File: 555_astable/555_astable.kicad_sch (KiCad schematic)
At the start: 10 parts, among them J1 Conn_01x02, J2 Conn_01x03, J3 Conn_01x02, SW1 SW_SPST, U1 NE555P

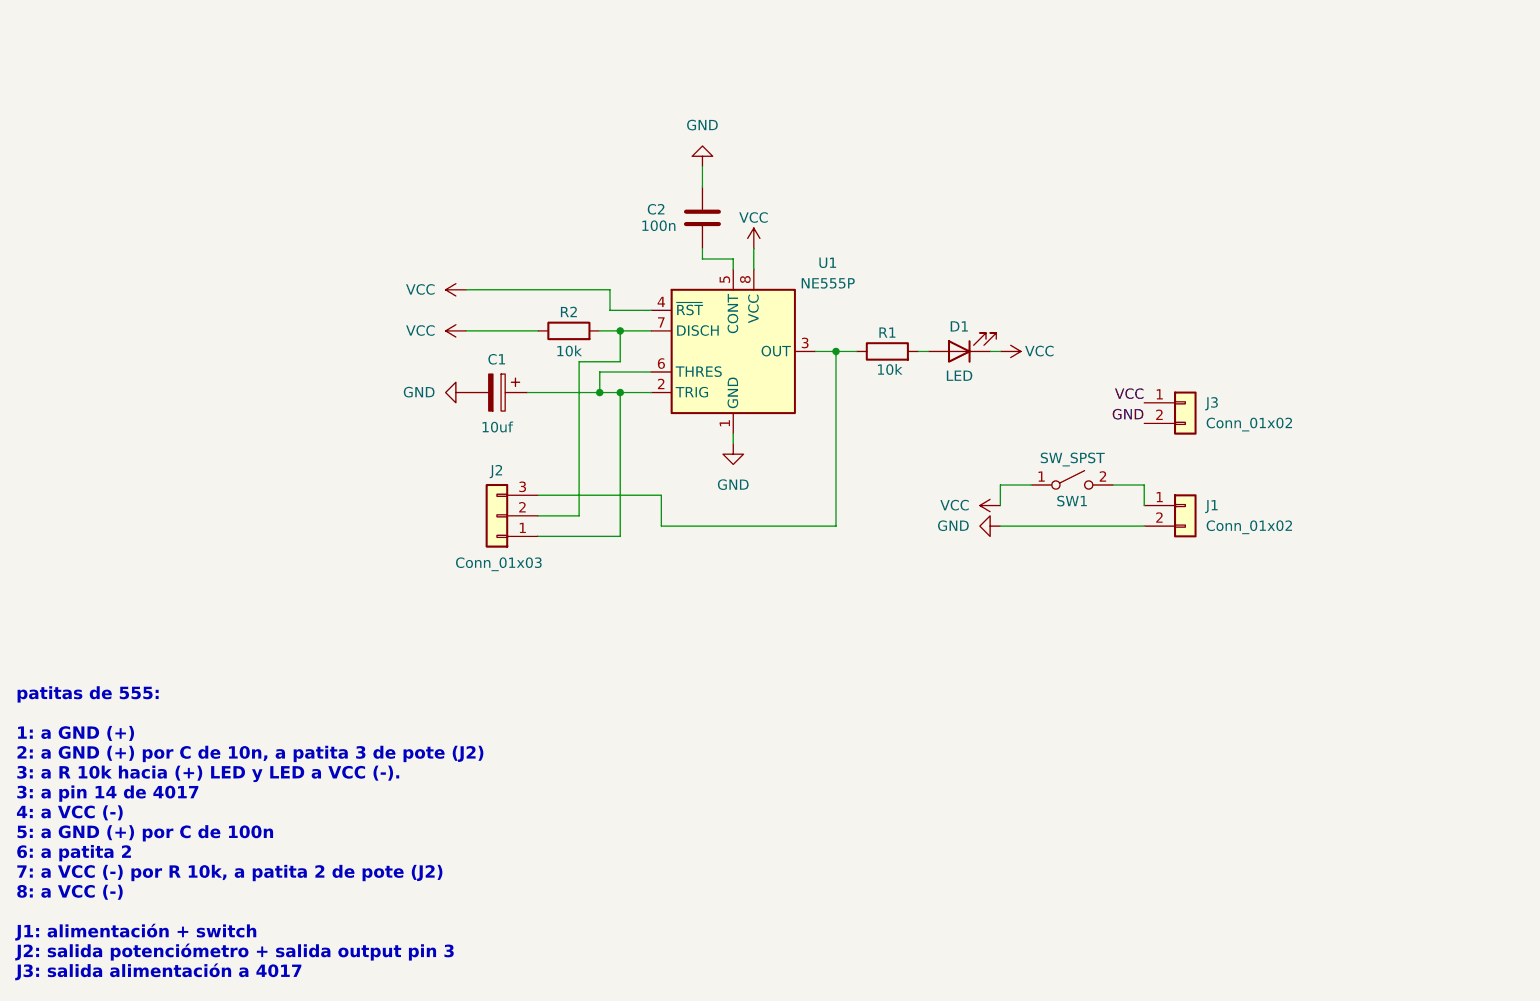
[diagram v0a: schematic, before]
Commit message: nueva version corregida de sch
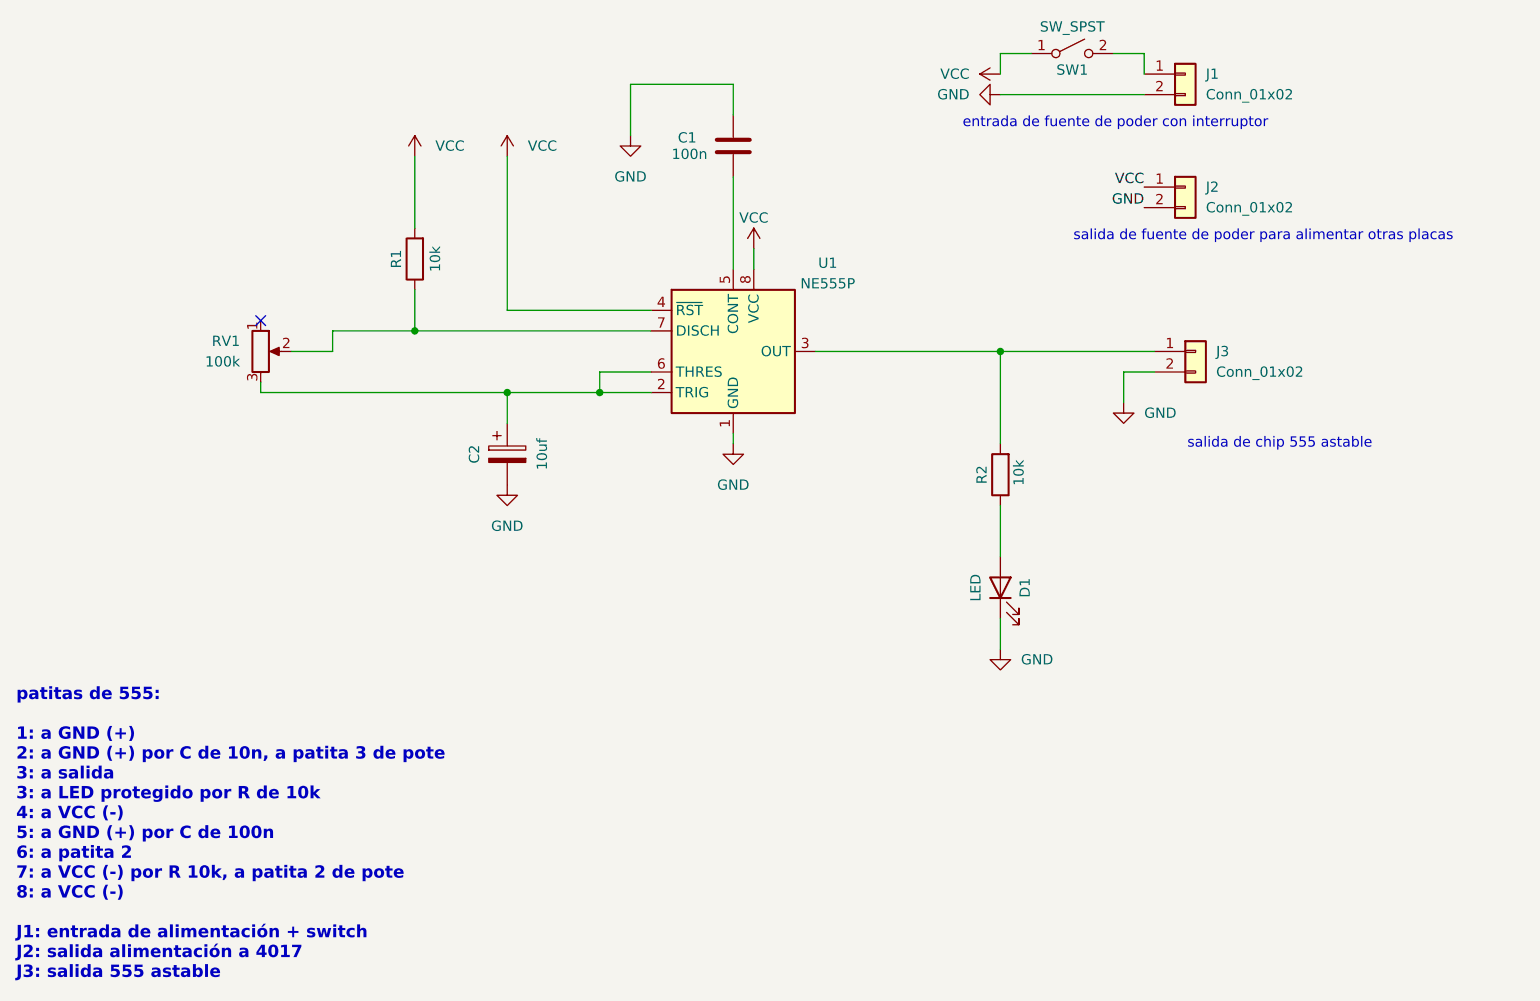
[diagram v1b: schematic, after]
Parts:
- removed C1: 10uf, Capacitor_THT:C_Radial_D5.0mm_H5.0mm_P2.00mm, symbol Device:C_Polarized
- removed C2: 100n, Capacitor_THT:C_Disc_D5.0mm_W2.5mm_P5.00mm, symbol Device:C
- removed J2: Conn_01x03, TerminalBlock:TerminalBlock_MaiXu_MX126-5.0-03P_1x03_P5.00mm, symbol Connector_Generic:Conn_01x03
- added C1: 100n, Capacitor_THT:C_Disc_D5.0mm_W2.5mm_P5.00mm, symbol Device:C
- added C2: 10uf, Capacitor_THT:C_Radial_D5.0mm_H5.0mm_P2.00mm, symbol Device:C_Polarized
- added J3: Conn_01x02, TerminalBlock:TerminalBlock_MaiXu_MX126-5.0-02P_1x02_P5.00mm, symbol Connector_Generic:Conn_01x02
- added RV1: 100k, TerminalBlock:TerminalBlock_MaiXu_MX126-5.0-02P_1x02_P5.00mm, symbol Device:R_Potentiometer
- renumbered J3 to J2
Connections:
- net GND: now also D1.1 (K), C1.1, C2.2, J3.2 (Pin_2)
- net VCC: now also R1.2; no longer D1.1 (K), R2.1
- net at U1.2 (TRIG), U1.6 (THRES): now also C2.1, RV1.3
- net at R1.1: now also U1.7 (DISCH), RV1.2; no longer U1.3 (OUT)
- net at U1.5 (CONT): now also C1.2
- net at R2.2: now also U1.3 (OUT), J3.1 (Pin_1); no longer U1.7 (DISCH)
- net at D1.2 (A): now also R2.1; no longer R1.2
- no-connect marks 0 -> 1
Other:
- note added: "entrada de fuente de poder con interruptor"
- note added: "patitas de 555: 1: a GND (+) 2: a GND (+) por C de 10n, a patita 3 de pote 3: a salida 3: a LED protegido por R de 10k 4: a VCC (-) 5: a GND (+) por C de 100n 6: a patita 2 7: a VCC (-) por R 10k, a patita 2 de pote 8: a VCC (-) J1: entrada de alimentación + switch J2: salida alimentación a 4017 J3: salida 555 astable"
- note added: "salida de chip 555 astable"
- note added: "salida de fuente de poder para alimentar otras placas"
- note removed: "patitas de 555: 1: a GND (+) 2: a GND (+) por C de 10n, a patita 3 de pote (J2) 3: a R 10k hacia (+) LED y LED a VCC (-). 3: a pin 14 de 4017 4: a VCC (-) 5: a GND (+) por C de 100n 6: a patita 2 7: a VCC (-) por R 10k, a patita 2 de pote (J2) 8: a VCC (-) J1: alimentación + switch J2: salida potenciómetro + salida output pin 3 J3: salida alimentación a 4017"
- moved on the sheet: J1, J2, SW1
